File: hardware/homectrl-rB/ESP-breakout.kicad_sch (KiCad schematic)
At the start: 3 parts, among them SW1 SW_RESET, SW2 SW_BOOT, U1 ESP32-S3-WROOM-1

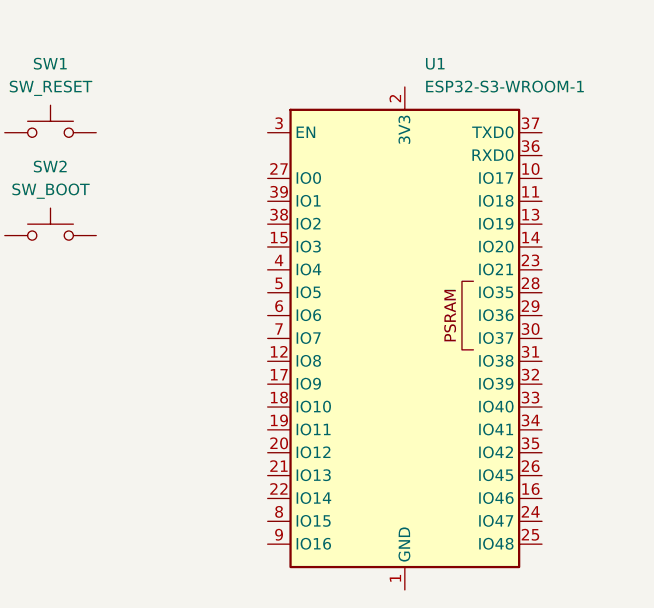
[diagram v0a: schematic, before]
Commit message: power circuitry
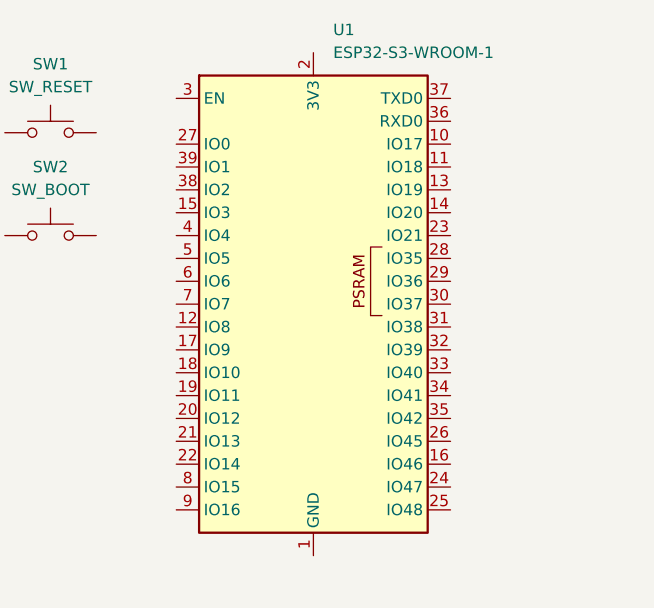
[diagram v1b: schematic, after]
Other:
- moved on the sheet: U1
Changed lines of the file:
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@@
 	(symbol
 		(lib_id "RF_Module:ESP32-S3-WROOM-1")
-		(at 134.62 87.63 0)
+		(at 124.46 83.82 0)
 		(unit 1)
 		(exclude_from_sim no)
@@
 		(fields_autoplaced yes)
 		(property "Reference" "U1"
-			(at 136.8141 57.15 0)
+			(at 126.6541 53.34 0)
 			(effects
 				(font
@@
 		)
 		(property "Value" "ESP32-S3-WROOM-1"
-			(at 136.8141 59.69 0)
+			(at 126.6541 55.88 0)
 			(effects
 				(font
@@
 		)
 		(property "Footprint" "RF_Module:ESP32-S3-WROOM-1"
-			(at 134.62 85.09 0)
+			(at 124.46 81.28 0)
 			(effects
 				(font
@@
 		)
 		(property "Datasheet" "https://www.espressif.com/sites/default/files/documentation/esp32-s3-wroom-1_wroom-1u_datasheet_en.pdf"
-			(at 134.62 87.63 0)
+			(at 124.46 83.82 0)
 			(effects
 				(font
@@
 		)
 		(property "Description" "RF Module, ESP32-S3 SoC, Wi-Fi 802.11b/g/n, Bluetooth, BLE, 32-bit, 3.3V, onboard antenna, SMD"
-			(at 134.62 87.63 0)
+			(at 124.46 83.82 0)
 			(effects
 				(font

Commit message: assign footprints
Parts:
- SW1, SW2: footprint (none) -> Button_Switch_THT:SW_PUSH_6mm
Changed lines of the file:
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@@
 			)
 		)
-		(property "Footprint" ""
+		(property "Footprint" "Button_Switch_THT:SW_PUSH_6mm"
 			(at 95.25 59.69 0)
 			(effects
@@
 			)
 		)
-		(property "Footprint" ""
+		(property "Footprint" "Button_Switch_THT:SW_PUSH_6mm"
 			(at 95.25 71.12 0)
 			(effects

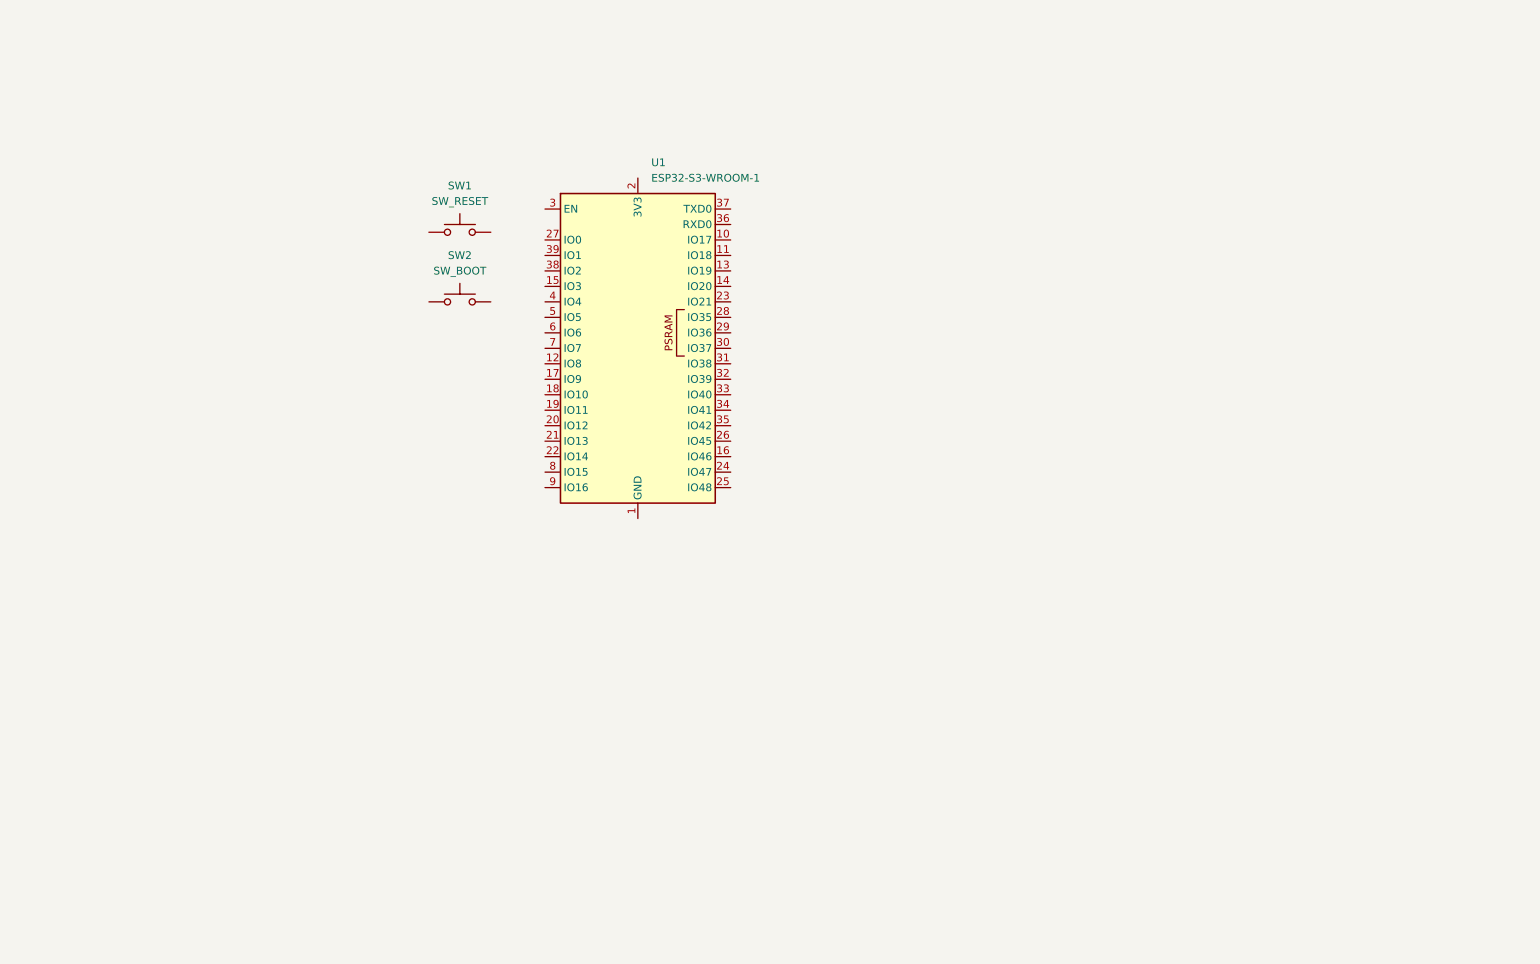
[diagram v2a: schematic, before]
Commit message: pmux & breakout circuitry
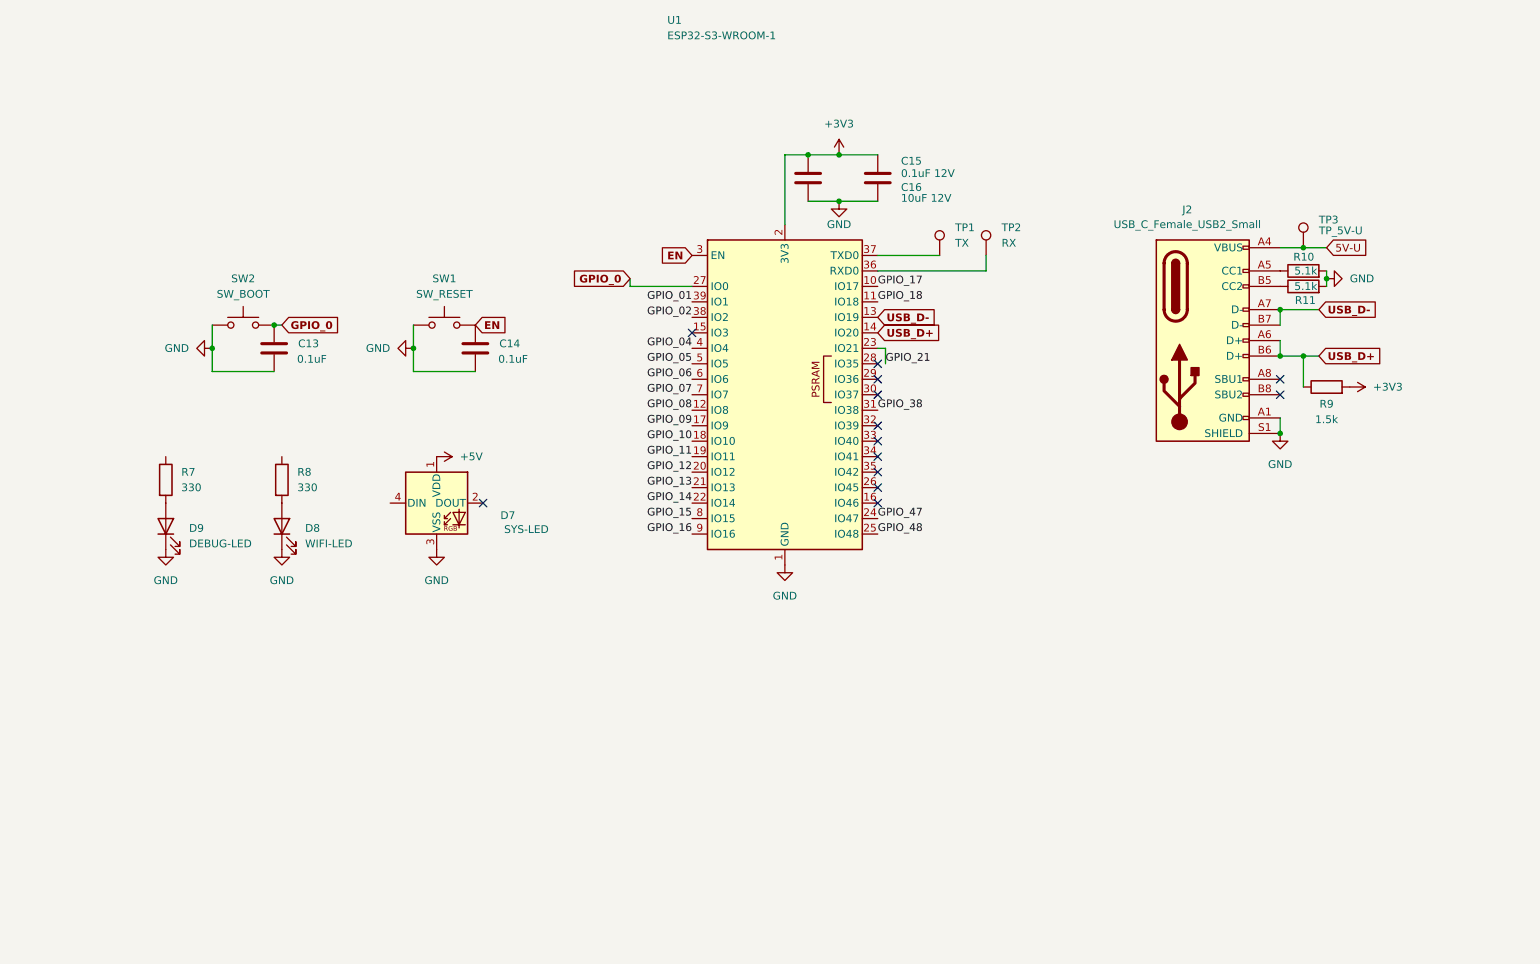
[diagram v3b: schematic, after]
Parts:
- added C13, C14: 0.1uF, Capacitor_SMD:C_0603_1608Metric, symbol Device:C
- added C15: 0.1uF 12V, Capacitor_SMD:C_0603_1608Metric, symbol Device:C
- added C16: 10uF 12V, Capacitor_SMD:C_0603_1608Metric, symbol Device:C
- added D7: SYS-LED, LED_SMD:LED_WS2812B_PLCC4_5.0x5.0mm_P3.2mm, symbol LED:WS2812B
- added D8: WIFI-LED, Diode_SMD:D_0805_2012Metric, symbol Device:LED
- added D9: DEBUG-LED, Diode_SMD:D_0805_2012Metric, symbol Device:LED
- added J2: USB_C_Female_USB2_Small, USBC-CONN:USB_C_DB-108PWB, symbol USB_C:USB_C_Female_USB2_Small
- added R10, R11: 5.1k, Resistor_SMD:R_0603_1608Metric, symbol Device:R
- added R7, R8: 330, Resistor_SMD:R_0402_1005Metric, symbol Device:R
- added R9: 1.5k, Resistor_SMD:R_0402_1005Metric, symbol Device:R
- added TP1: TX, TestPoint:TestPoint_Pad_1.0x1.0mm, symbol Connector:TestPoint
- added TP2: RX, TestPoint:TestPoint_Pad_1.0x1.0mm, symbol Connector:TestPoint
- added TP3: TP_5V-U, TestPoint:TestPoint_Pad_1.0x1.0mm, symbol Connector:TestPoint
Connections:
- net GND: now reaches SW1.1
- net GND: now also SW2.1, U1.1 (GND), U1.40 (GND), U1.41 (GND), C13.1, C14.1, C15.2, C16.2, D7.3 (VSS), D8.1 (K), D9.1 (K), J2.A1 (GND), J2.A12 (GND), J2.B1 (GND), J2.B12 (GND), J2.S1 (SHIELD), R10.2, R11.2
- net EN: now reaches SW1.2
- net EN: now also U1.3 (EN), C14.2
- net GPIO_0: now reaches SW2.2
- net GPIO_0: now also U1.27 (IO0), C13.2
- net GPIO_17: now reaches U1.10 (IO17)
- net GPIO_18: now reaches U1.11 (IO18)
- net GPIO_08: now reaches U1.12 (IO8)
- net USB_D-: now reaches U1.13 (IO19)
- net USB_D-: now also J2.A7 (D-), J2.B7 (D-)
- net USB_D+: now reaches U1.14 (IO20)
- net USB_D+: now also J2.A6 (D+), J2.B6 (D+), R9.1
- net GPIO_09: now reaches U1.17 (IO9)
- net GPIO_10: now reaches U1.18 (IO10)
- net GPIO_11: now reaches U1.19 (IO11)
- net +3V3: now reaches U1.2 (3V3)
- net +3V3: now also C15.1, C16.1, R9.2
- net GPIO_12: now reaches U1.20 (IO12)
- net GPIO_13: now reaches U1.21 (IO13)
- net GPIO_14: now reaches U1.22 (IO14)
- net GPIO_21: now reaches U1.23 (IO21)
- net GPIO_47: now reaches U1.24 (IO47)
- net GPIO_48: now reaches U1.25 (IO48)
- net GPIO_38: now reaches U1.31 (IO38)
- net at U1.36 (RXD0): now also TP2.1
- net at U1.37 (TXD0): now also TP1.1
- net GPIO_02: now reaches U1.38 (IO2)
- net GPIO_01: now reaches U1.39 (IO1)
- net GPIO_04: now reaches U1.4 (IO4)
- net GPIO_05: now reaches U1.5 (IO5)
- net GPIO_06: now reaches U1.6 (IO6)
- net GPIO_07: now reaches U1.7 (IO7)
- net GPIO_15: now reaches U1.8 (IO15)
- net GPIO_16: now reaches U1.9 (IO16)
- new net: D9.2 (A), R7.2
- new net: J2.A5 (CC1), R10.1
- new net: D8.2 (A), R8.2
- new net: J2.B5 (CC2), R11.1
- new net +5V: D7.1 (VDD)
- new net 5V-U: J2.A4 (VBUS), J2.A9 (VBUS), J2.B4 (VBUS), J2.B9 (VBUS), TP3.1
- no-connect marks 0 -> 13
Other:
- moved on the sheet: SW1, SW2, U1

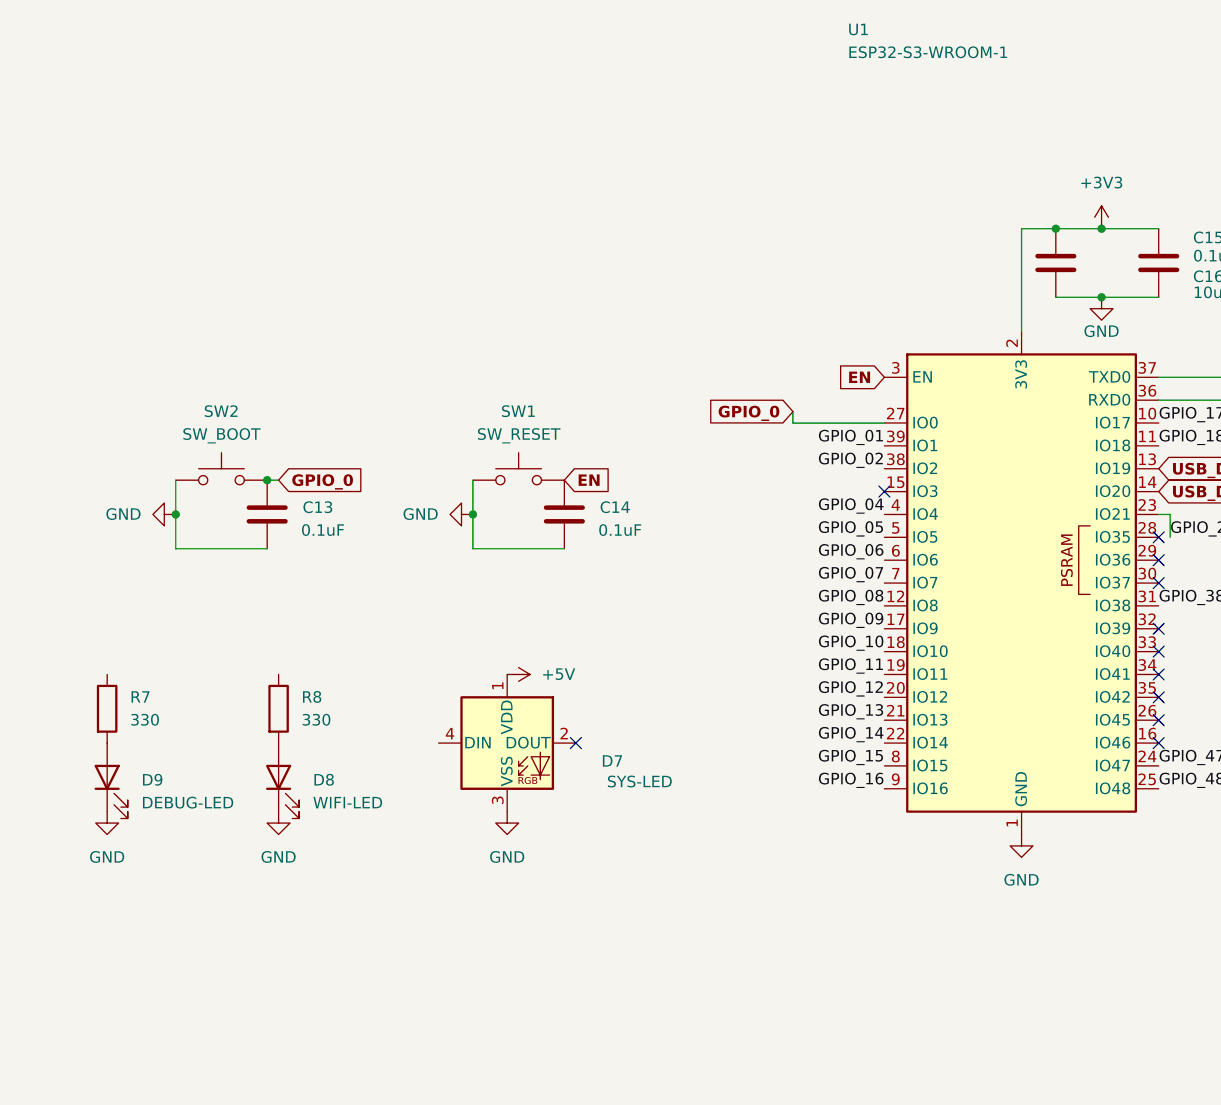
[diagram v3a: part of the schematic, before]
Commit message: sensing circuitry
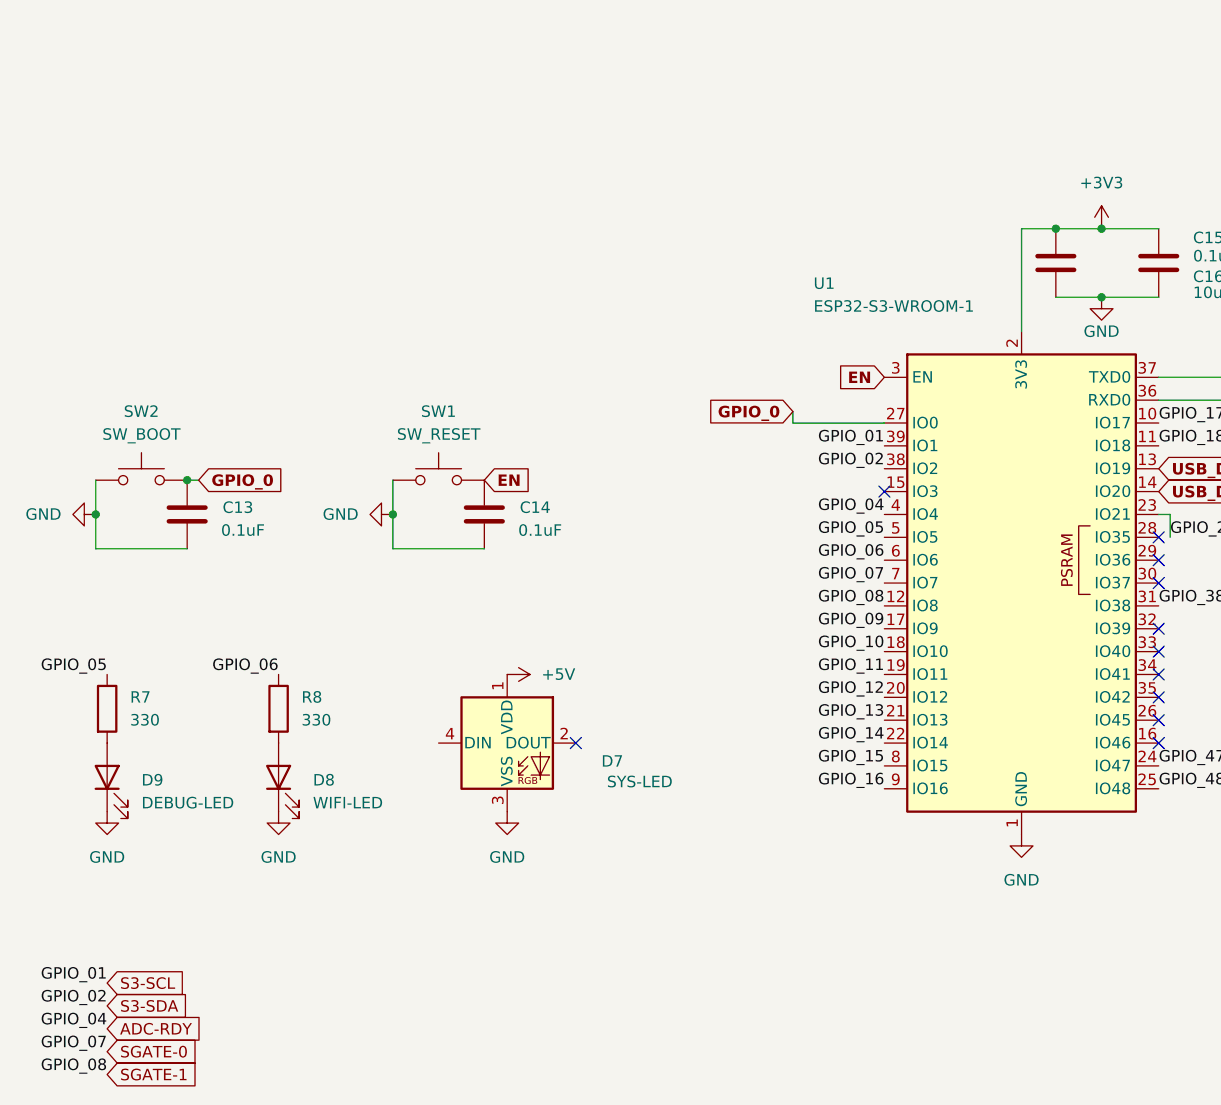
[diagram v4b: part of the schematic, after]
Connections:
- net GPIO_05: now also R7.1
- net GPIO_06: now also R8.1
- net GPIO_01 renamed S3-SCL
- net GPIO_02 renamed S3-SDA
- net GPIO_04 renamed ADC-RDY
- net GPIO_07 renamed SGATE-0
- net GPIO_08 renamed SGATE-1
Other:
- moved on the sheet: C13, C14, SW1, SW2

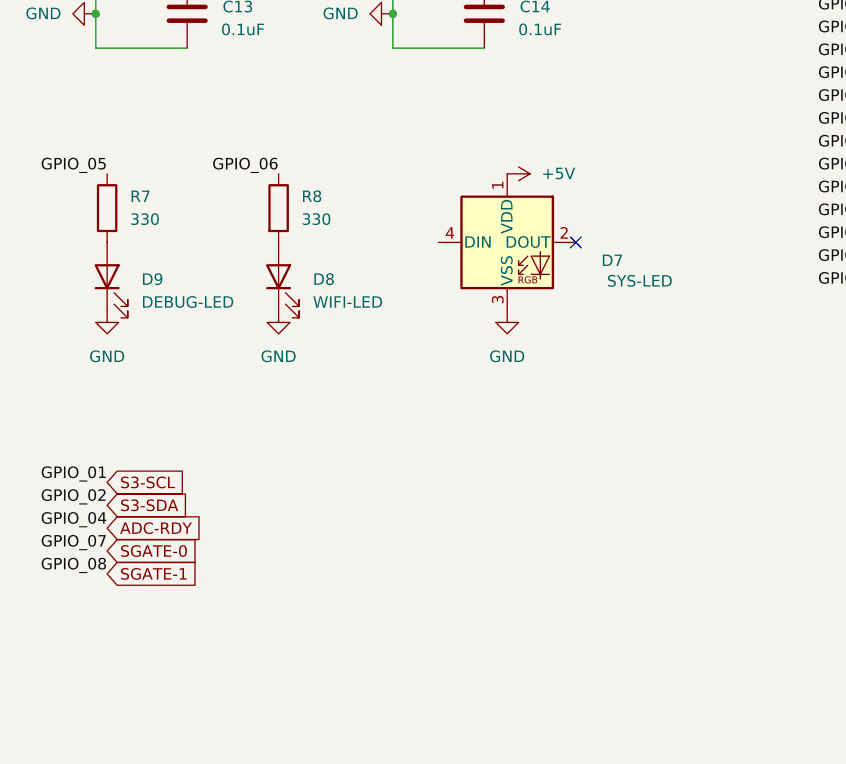
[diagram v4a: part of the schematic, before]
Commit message: stepper driver circuitry
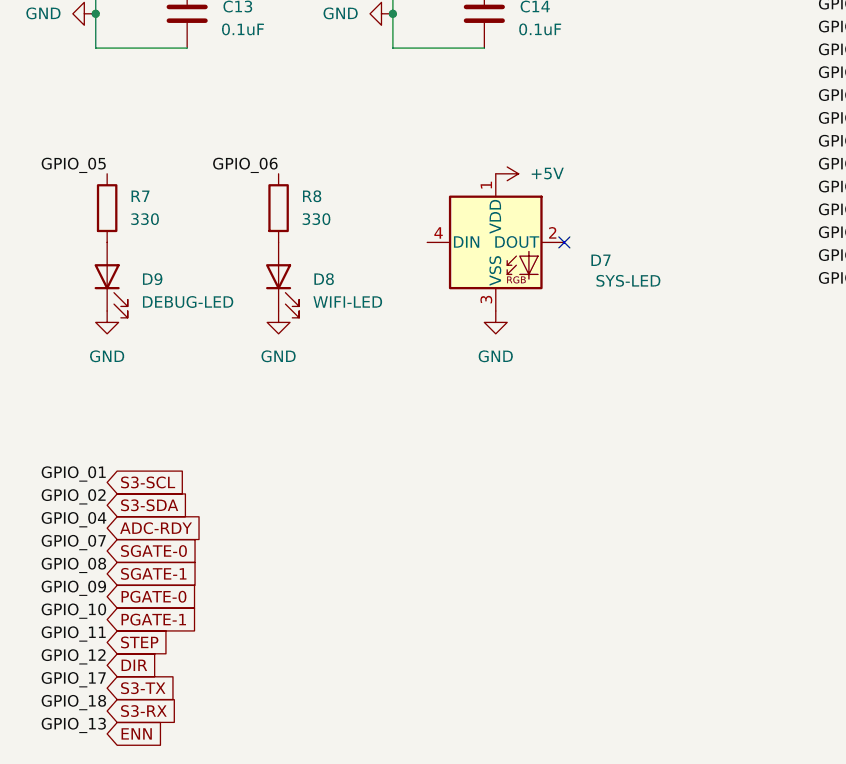
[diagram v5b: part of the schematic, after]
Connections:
- net GPIO_09 renamed PGATE-0
- net GPIO_10 renamed PGATE-1
- net GPIO_11 renamed STEP
- net GPIO_12 renamed DIR
- net GPIO_13 renamed ENN
- net GPIO_17 renamed S3-TX
- net GPIO_18 renamed S3-RX
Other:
- moved on the sheet: D7
